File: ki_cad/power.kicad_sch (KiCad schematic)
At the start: 14 parts, among them Q6 Q_NMOS, U3 SY81051

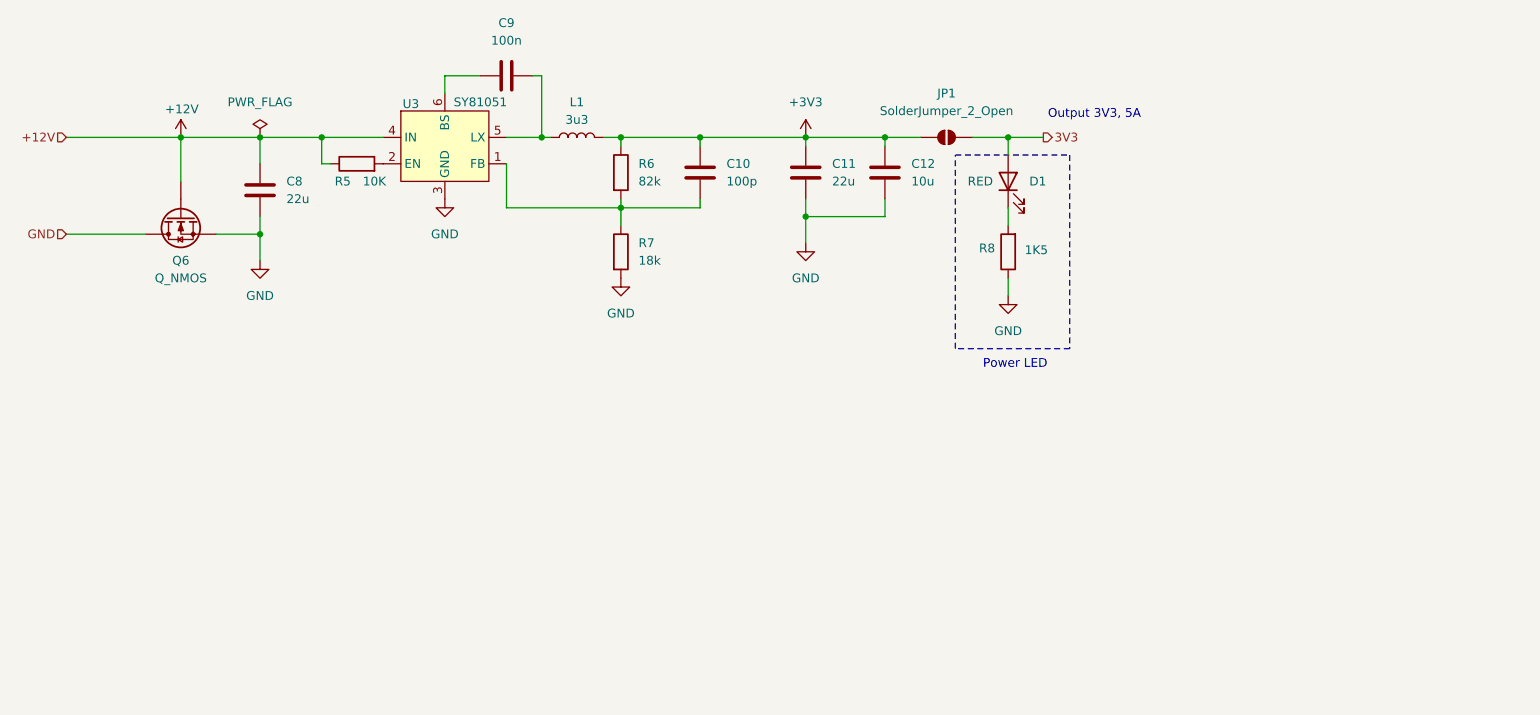
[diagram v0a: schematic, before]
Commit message: update after feedback (purchased)
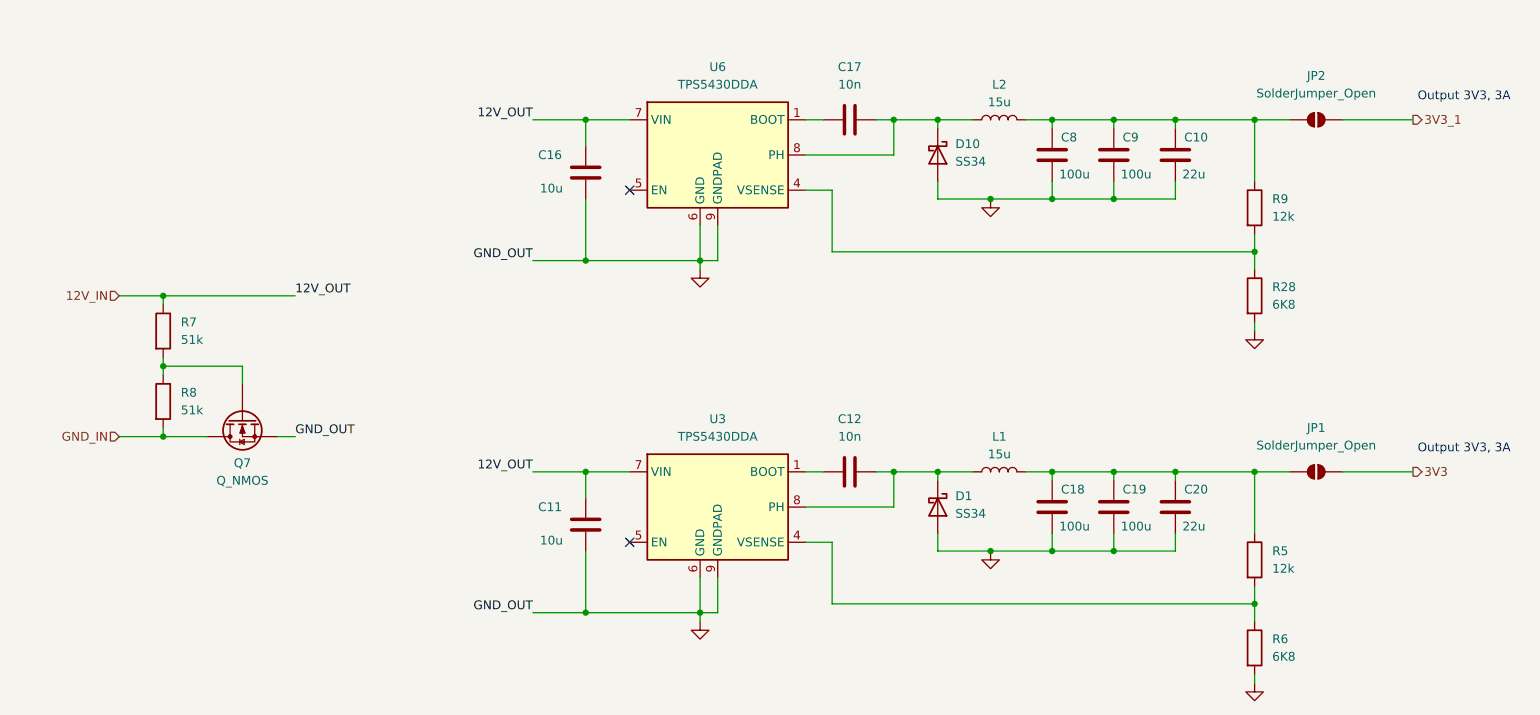
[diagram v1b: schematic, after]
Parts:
- removed D1: RED, Diode_SMD:D_0603_1608Metric, symbol Device:LED
- removed Q6: Q_NMOS, Custom:SOT-23-3, symbol Device:Q_NMOS
- removed U3: SY81051, Package_TO_SOT_SMD:TSOT-23-6, symbol basic_parts_MICH:SY8105I
- added C16: 10u, Capacitor_SMD:C_0805_2012Metric, symbol Device:C
- added C17: 10n, Capacitor_SMD:C_0805_2012Metric, symbol Device:C
- added C18, C19: 100u, Capacitor_SMD:C_1206_3216Metric, symbol Device:C
- added C20: 22u, Capacitor_SMD:C_0805_2012Metric, symbol Device:C
- added D1, D10: SS34, Diode_SMD:D_SMA, symbol Device:D_Schottky
- added JP2: SolderJumper_Open, Jumper:SolderJumper-2_P1.3mm_Open_RoundedPad1.0x1.5mm, symbol Jumper:SolderJumper_2_Open
- added L2: 15u, Custom:CYA0630, symbol Device:L
- added Q7: Q_NMOS, Custom:SOT-23-3, symbol Device:Q_NMOS
- added R28: 6K8, Resistor_SMD:R_0603_1608Metric, symbol Device:R
- added R9: 12k, Resistor_SMD:R_0603_1608Metric, symbol Device:R
- added U3, U6: TPS5430DDA, Package_SO:TI_SO-PowerPAD-8_ThermalVias, symbol Regulator_Switching:TPS5430DDA
- C10: value 100p -> 22u; footprint Resistor_SMD:R_0603_1608Metric -> Capacitor_SMD:C_0805_2012Metric; JLCPCB Part # C14858 -> C45783
- C11: value 22u -> 10u; footprint Resistor_SMD:R_0603_1608Metric -> Capacitor_SMD:C_0805_2012Metric; JLCPCB Part # C59461 -> C15850
- C12: value 10u -> 10n; footprint Capacitor_SMD:C_0402_1005Metric -> Capacitor_SMD:C_0805_2012Metric; JLCPCB Part # C15525 -> C1710
- C8: value 22u -> 100u; footprint Resistor_SMD:R_0603_1608Metric -> Capacitor_SMD:C_1206_3216Metric; JLCPCB Part # C59461 -> C15008
- C9: value 100n -> 100u; footprint Capacitor_SMD:C_0402_1005Metric -> Capacitor_SMD:C_1206_3216Metric; JLCPCB Part # C307331 -> C15008
- JP1: value SolderJumper_2_Open -> SolderJumper_Open
- L1: value 3u3 -> 15u; footprint Inductor_SMD:L_KOHERelec_MDA5030 -> Custom:CYA0630; Field5 (none) -> C5189959; JLCPCB Part # C2847476 -> C5189959
- R5: value 10K -> 12k; footprint Resistor_SMD:R_0805_2012Metric -> Resistor_SMD:R_0603_1608Metric; JLCPCB Part # C17414 -> C22790
- R6: value 82k -> 6K8; footprint Resistor_SMD:R_0201_0603Metric -> Resistor_SMD:R_0603_1608Metric; JLCPCB Part # C23254 -> C23212
- R7: value 18k -> 51k; footprint Resistor_SMD:R_0201_0603Metric -> Resistor_SMD:R_0603_1608Metric; JLCPCB Part # C25810 -> C23196
- R8: value 1K5 -> 51k; footprint Resistor_SMD:R_0201_0603Metric -> Resistor_SMD:R_0603_1608Metric; JLCPCB Part # C22843 -> C23196
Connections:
- net GND: now also C10.2, C9.2, R6.2, C16.2, C18.2, C19.2, C20.2, D1.2 (A), D10.2 (A), Q7.S, R28.2, U3.6 (GND), U3.9 (GNDPAD), U6.6 (GND), U6.9 (GNDPAD); no longer C12.2, R7.2, R8.1
- net at L1.1: now also C12.2, D1.1 (K), U3.8 (PH); no longer C9.2
- net at R5.2: now also R6.1, U3.4 (VSENSE)
- net GND_IN: now reaches R8.2
- net GND_IN: now also Q7.D
- net at C9.1: now also C10.1, C8.1, JP2.1 (A), L2.2, R9.1
- net +12V: no longer names the net of R5.1
- net +12V: now also JP1.1 (A), L1.2, C18.1, C19.1, C20.1; no longer C8.1
- removed net +3V3: C10.1, C11.1, C12.1, JP1.1 (A), L1.2, R6.1
- new net: C17.2, D10.1 (K), L2.1, U6.8 (PH)
- new net: Q7.G, R7.2, R8.1
- new net: R28.1, R9.2, U6.4 (VSENSE)
- new net: C12.1, U3.1 (BOOT)
- new net: C17.1, U6.1 (BOOT)
- new net 12V_IN: C11.1, C16.1, R7.1, U3.7 (VIN), U6.7 (VIN)
- new net 3V3_1: JP2.2 (B)
- no-connect marks 0 -> 2
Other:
- note added: "Output 3V3, 3A"
- note removed: "Output 3V3, 5A"
- note removed: "Power LED"

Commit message: update code
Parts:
- JP1, JP2: footprint Jumper:SolderJumper-2_P1.3mm_Open_RoundedPad1.0x1.5mm -> Jumper:SolderJumper-2_P1.3mm_Open_TrianglePad1.0x1.5mm
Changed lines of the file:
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@@
 		)
 		(instances
-			(project ""
+			(project "pwm_board"
 				(path "/71ddf0e9-b3bd-413d-a31e-e27757e0e466/86d7eb10-d134-4986-b82a-cc819e39ad23"
 					(reference "L2")
@@
 		)
 		(instances
-			(project ""
+			(project "pwm_board"
 				(path "/71ddf0e9-b3bd-413d-a31e-e27757e0e466/86d7eb10-d134-4986-b82a-cc819e39ad23"
 					(reference "D10")
@@
 		)
 		(instances
-			(project ""
+			(project "pwm_board"
 				(path "/71ddf0e9-b3bd-413d-a31e-e27757e0e466/86d7eb10-d134-4986-b82a-cc819e39ad23"
 					(reference "C17")
@@
 			)
 		)
-		(property "Footprint" "Jumper:SolderJumper-2_P1.3mm_Open_RoundedPad1.0x1.5mm"
+		(property "Footprint" "Jumper:SolderJumper-2_P1.3mm_Open_TrianglePad1.0x1.5mm"
 			(at 213.36 104.14 0)
 			(effects
@@
 		)
 		(instances
-			(project ""
+			(project "pwm_board"
 				(path "/71ddf0e9-b3bd-413d-a31e-e27757e0e466/86d7eb10-d134-4986-b82a-cc819e39ad23"
 					(reference "C16")
@@
 		)
 		(instances
-			(project ""
+			(project "pwm_board"
 				(path "/71ddf0e9-b3bd-413d-a31e-e27757e0e466/86d7eb10-d134-4986-b82a-cc819e39ad23"
 					(reference "U6")
@@
 			)
 		)
-		(property "Footprint" "Jumper:SolderJumper-2_P1.3mm_Open_RoundedPad1.0x1.5mm"
+		(property "Footprint" "Jumper:SolderJumper-2_P1.3mm_Open_TrianglePad1.0x1.5mm"
 			(at 213.36 53.34 0)
 			(effects

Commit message: copy arduino lib for PCA9635
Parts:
- JP1, JP2: footprint Jumper:SolderJumper-2_P1.3mm_Open_TrianglePad1.0x1.5mm -> Jumper:SolderJumper-2_P1.3mm_Open_RoundedPad1.0x1.5mm
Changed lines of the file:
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@@
 			)
 		)
-		(property "Footprint" "Jumper:SolderJumper-2_P1.3mm_Open_TrianglePad1.0x1.5mm"
+		(property "Footprint" "Jumper:SolderJumper-2_P1.3mm_Open_RoundedPad1.0x1.5mm"
 			(at 213.36 104.14 0)
 			(effects
@@
 			)
 		)
-		(property "Footprint" "Jumper:SolderJumper-2_P1.3mm_Open_TrianglePad1.0x1.5mm"
+		(property "Footprint" "Jumper:SolderJumper-2_P1.3mm_Open_RoundedPad1.0x1.5mm"
 			(at 213.36 53.34 0)
 			(effects
